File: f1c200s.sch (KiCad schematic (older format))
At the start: 21 parts, among them J1 Conn_02x14_Odd_Even, J13 Conn_01x06_Male, J2 Conn_01x04_Male, J3 Conn_01x07_Male, J4 Conn_02x03_Odd_Even, J5 Conn_01x03_Male, J6 Conn_01x04_Male, J8 Conn_01x06_Male, J9 Conn_01x01_Male, SW1 SW_Push, U2 F1C100s, Y1 24MHz

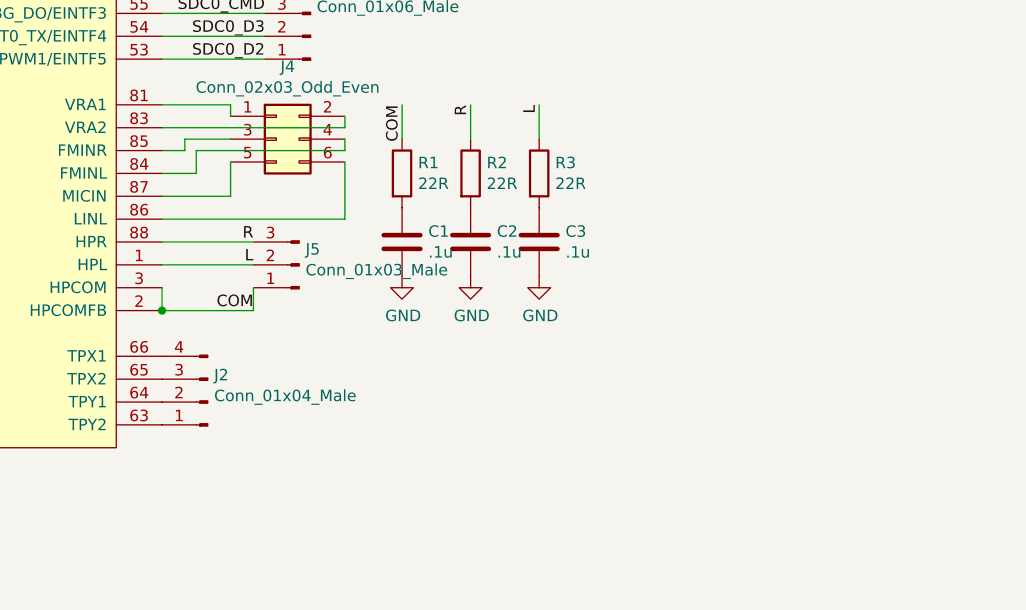
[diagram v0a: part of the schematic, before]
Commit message: second rev of crap board
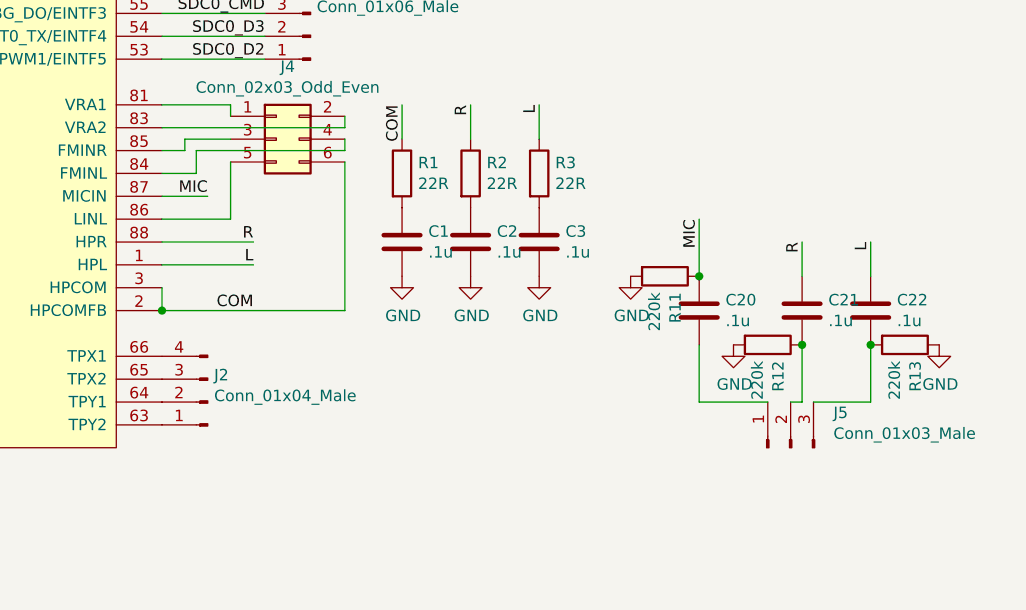
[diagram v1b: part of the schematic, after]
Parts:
- added C20, C21, C22: .1u, Capacitor_SMD:C_0603_1608Metric_Pad1.05x0.95mm_HandSolder, symbol Device:C
- added R11, R12, R13: 220k, Capacitor_SMD:C_0603_1608Metric_Pad1.05x0.95mm_HandSolder, symbol Device:R
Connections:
- net COM: now also J4.6 (Pin_6); no longer J5.1 (Pin_1)
- net GND: now also R11.2, R12.2, R13.1
- net L: now also C22.1; no longer J5.2 (Pin_2)
- net R: now also C21.1; no longer J5.3 (Pin_3)
- net at U2.86 (LINL): now also J4.5 (Pin_5); no longer J4.6 (Pin_6)
- net MIC: now reaches U2.87 (MICIN)
- net MIC: now also C20.1, R11.1; no longer J4.5 (Pin_5)
- new net: C20.2, J5.1 (Pin_1)
- new net: C22.2, J5.3 (Pin_3), R13.2
- new net: C21.2, J5.2 (Pin_2), R12.1
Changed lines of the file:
@@
 EESchema Schematic File Version 4
-EELAYER 30 0
+LIBS:f1c200s-cache
+EELAYER 26 0
 EELAYER END
 $Descr A4 11693 8268
@@
 Text Label 7250 4100 2    50   ~ 0
 R
-Text Label 7250 4400 2    50   ~ 0
-COM
 $Comp
 L power:GND #PWR0101
@@
 Wire Wire Line
 	7650 3700 7650 3650
-Wire Wire Line
-	7150 3900 6850 3900
-Wire Wire Line
-	7150 3750 7150 3900
-Wire Wire Line
-	6850 4000 7650 4000
-Wire Wire Line
-	7650 4000 7650 3750
-Wire Wire Line
-	7250 4400 6850 4400
 Connection ~ 6850 4400
 $Comp
+L Device:R R11
+U 1 1 5F45AC07
+P 9050 4250
+F 0 "R11" H 9120 4296 50  0000 L CNN
+F 1 "220k" H 9120 4205 50  0000 L CNN
+F 2 "Capacitor_SMD:C_0603_1608Metric_Pad1.05x0.95mm_HandSolder" V 8980 4250 50  0001 C CNN
+F 3 "~" H 9050 4250 50  0001 C CNN
+	1    9050 4250
+	0    1    1    0
+$EndComp
+$Comp
+L Device:C C20
+U 1 1 5F45AC0E
+P 9200 4400
+F 0 "C20" H 9315 4446 50  0000 L CNN
+F 1 ".1u" H 9315 4355 50  0000 L CNN
+F 2 "Capacitor_SMD:C_0603_1608Metric_Pad1.05x0.95mm_HandSolder" H 9238 4250 50  0001 C CNN
+F 3 "~" H 9200 4400 50  0001 C CNN
+	1    9200 4400
+	1    0    0    -1
+$EndComp
+$Comp
+L Device:C C21
+U 1 1 5F45AC1C
+P 9650 4400
+F 0 "C21" H 9765 4446 50  0000 L CNN
+F 1 ".1u" H 9765 4355 50  0000 L CNN
+F 2 "Capacitor_SMD:C_0603_1608Metric_Pad1.05x0.95mm_HandSolder" H 9688 4250 50  0001 C CNN
+F 3 "~" H 9650 4400 50  0001 C CNN
+	1    9650 4400
+	1    0    0    -1
+$EndComp
+$Comp
+L Device:R R12
+U 1 1 5F45AC23
+P 9500 4550
+F 0 "R12" H 9570 4596 50  0000 L CNN
+F 1 "220k" H 9570 4505 50  0000 L CNN
+F 2 "Capacitor_SMD:C_0603_1608Metric_Pad1.05x0.95mm_HandSolder" V 9430 4550 50  0001 C CNN
+F 3 "~" H 9500 4550 50  0001 C CNN
+	1    9500 4550
+	0    1    1    0
+$EndComp
+$Comp
+L Device:C C22
+U 1 1 5F45AC2A
+P 9950 4400
+F 0 "C22" H 10065 4446 50  0000 L CNN
+F 1 ".1u" H 10065 4355 50  0000 L CNN
+F 2 "Capacitor_SMD:C_0603_1608Metric_Pad1.05x0.95mm_HandSolder" H 9988 4250 50  0001 C CNN
+F 3 "~" H 9950 4400 50  0001 C CNN
+	1    9950 4400
+	1    0    0    -1
+$EndComp
+$Comp
+L power:GND #PWR0170
+U 1 1 5F45AC31
+P 8900 4250
+F 0 "#PWR0170" H 8900 4000 50  0001 C CNN
+F 1 "GND" H 8905 4077 50  0000 C CNN
+F 2 "" H 8900 4250 50  0001 C CNN
+F 3 "" H 8900 4250 50  0001 C CNN
+	1    8900 4250
+	1    0    0    -1
+$EndComp
+$Comp
+L power:GND #PWR0171
+U 1 1 5F45AC37
+P 9350 4550
+F 0 "#PWR0171" H 9350 4300 50  0001 C CNN
+F 1 "GND" H 9355 4377 50  0000 C CNN
+F 2 "" H 9350 4550 50  0001 C CNN
+F 3 "" H 9350 4550 50  0001 C CNN
+	1    9350 4550
+	1    0    0    -1
+$EndComp
+Wire Wire Line
+	9650 4250 9650 4100
+Wire Wire Line
+	9950 4250 9950 4100
+$Comp
+L power:GND #PWR0172
+U 1 1 5F45AC40
+P 10250 4550
+F 0 "#PWR0172" H 10250 4300 50  0001 C CNN
+F 1 "GND" H 10255 4377 50  0000 C CNN
+F 2 "" H 10250 4550 50  0001 C CNN
+F 3 "" H 10250 4550 50  0001 C CNN
+	1    10250 4550
+	1    0    0    -1
+$EndComp
+Text Label 9950 4100 3    50   ~ 0
+L
+Text Label 9650 4100 3    50   ~ 0
+R
+Text Label 7250 4400 2    50   ~ 0
+COM
+Wire Wire Line
+	6850 4400 7650 4400
+Wire Wire Line
+	7650 3750 7650 4400
+$Comp
+L Device:R R13
+U 1 1 5F45AC15
+P 10100 4550
+F 0 "R13" H 10170 4596 50  0000 L CNN
+F 1 "220k" H 10170 4505 50  0000 L CNN
+F 2 "Capacitor_SMD:C_0603_1608Metric_Pad1.05x0.95mm_HandSolder" V 10030 4550 50  0001 C CNN
+F 3 "~" H 10100 4550 50  0001 C CNN
+	1    10100 4550
+	0    1    1    0
+$EndComp
+Wire Wire Line
+	6850 4000 7150 4000
+Wire Wire Line
+	7150 3750 7150 4000
+Wire Wire Line
+	6850 3900 7050 3900
+Text Label 7050 3900 2    50   ~ 0
+MIC
+Wire Wire Line
+	9200 4250 9200 4000
+Connection ~ 9200 4250
+Text Label 9200 4000 3    50   ~ 0
+MIC
+$Comp
 L Connector:Conn_01x03_Male J5
-U 1 1 5F77A1B9
-P 7450 4200
-F 0 "J5" H 7422 4132 50  0000 R CNN
-F 1 "Conn_01x03_Male" H 7422 4223 50  0000 R CNN
-F 2 "Connector_PinHeader_2.54mm:PinHeader_1x03_P2.54mm_Vertical" H 7450 4200 50  0001 C CNN
-F 3 "~" H 7450 4200 50  0001 C CNN
-	1    7450 4200
-	-1   0    0    1
-$EndComp
-Wire Wire Line
-	7250 4400 7250 4300
+U 1 1 5F491BF7
+P 9600 5000
+F 0 "J5" V 9753 4813 50  0000 R CNN
+F 1 "Conn_01x03_Male" V 9662 4813 50  0000 R CNN
+F 2 "Connector_PinHeader_2.54mm:PinHeader_1x03_P2.54mm_Vertical" H 9600 5000 50  0001 C CNN
+F 3 "~" H 9600 5000 50  0001 C CNN
+	1    9600 5000
+	0    -1   -1   0
+$EndComp
+Wire Wire Line
+	9600 4800 9650 4800
+Wire Wire Line
+	9650 4800 9650 4550
+Connection ~ 9650 4550
+Wire Wire Line
+	9700 4800 9950 4800
+Wire Wire Line
+	9950 4800 9950 4550
+Connection ~ 9950 4550
+Wire Wire Line
+	9500 4800 9200 4800
+Wire Wire Line
+	9200 4800 9200 4550
 $EndSCHEMATC
